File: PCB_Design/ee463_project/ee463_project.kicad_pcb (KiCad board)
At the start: 2 copper layers, 159.3 x 123.2 mm, 25 parts, among them Q1 C2M0080120D, U1 TLP250, U2 L7808, U3 ACS712xLCTR-30A

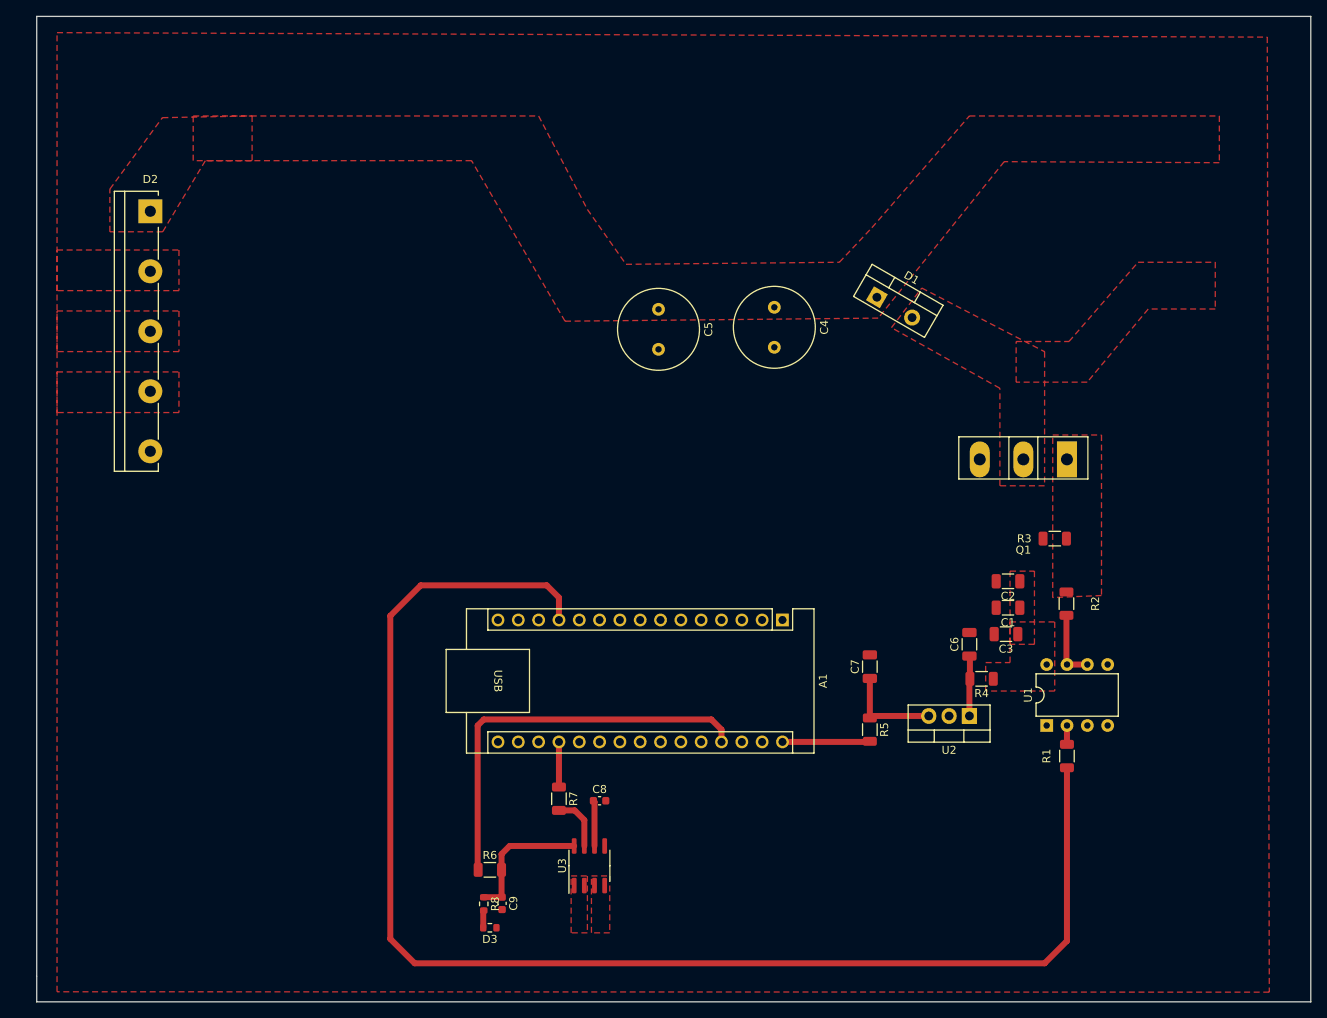
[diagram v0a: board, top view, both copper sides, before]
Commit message: PCB Design Updated
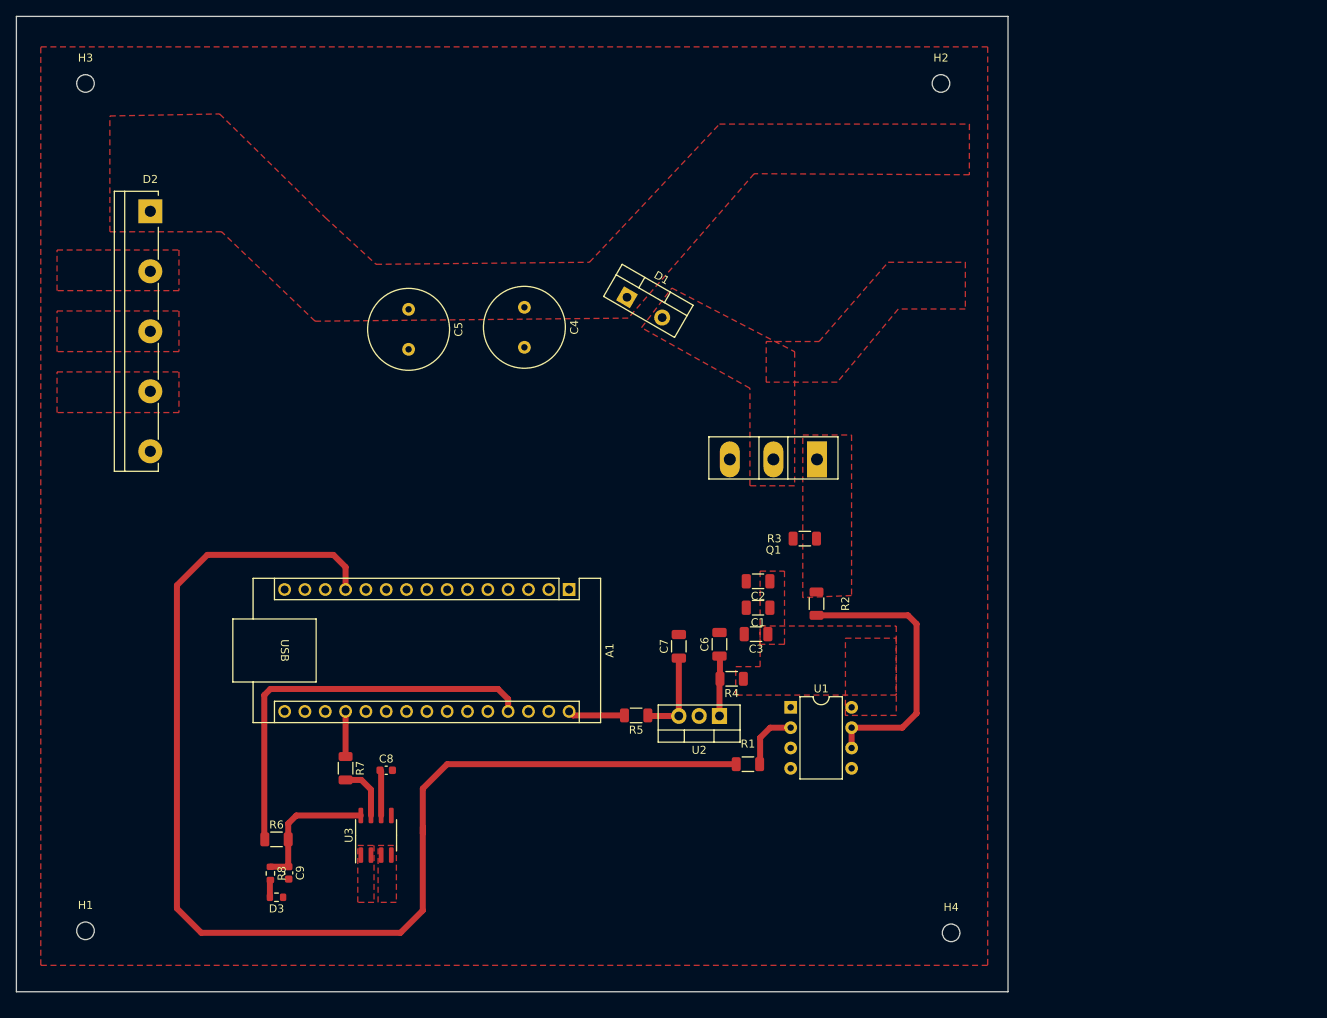
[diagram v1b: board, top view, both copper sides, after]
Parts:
- added H1: MountingHole, MountingHole:MountingHole_2.2mm_M2, F.Cu at (54.4, 133.4)
- added H2: MountingHole, MountingHole:MountingHole_2.2mm_M2, F.Cu at (161.3, 27.4)
- added H3: MountingHole, MountingHole:MountingHole_2.2mm_M2, F.Cu at (54.4, 27.4)
- added H4: MountingHole, MountingHole:MountingHole_2.2mm_M2, F.Cu at (162.6, 133.6)
- moved R1 39.9 mm to (137.2, 112.5), turned to 0 degrees
- moved U1 32.1 mm to (142.5, 105.4), turned to 0 degrees
- moved C3 31.2 mm to (138.2, 96.3)
- moved Q1 31.2 mm to (145.8, 74.4)
- moved R3 31.2 mm to (144.3, 84.3)
- moved R4 31.2 mm to (135.1, 101.9)
- moved C1 31.2 mm to (138.4, 93.0)
- moved C2 31.2 mm to (138.4, 89.7)
- moved C4 31.2 mm to (109.2, 55.4)
- moved C5 31.2 mm to (94.7, 55.7)
- moved C6 31.2 mm to (133.6, 97.5)
- moved D1 31.2 mm to (122.0, 54.2)
- moved R2 31.2 mm to (145.7, 92.5)
- moved U2 31.2 mm to (133.6, 106.5)
- moved R5 29.3 mm to (123.2, 106.4), turned to 180 degrees
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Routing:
- net Net-(R2-Pad1): track 8.72 -> 35.5 mm
- net PWM: track 175.1 -> 156.1 mm
- net Net-(R1-Pad2): track 2.36 -> 7.67 mm
- net V_in_arduino: track 11.0 -> 7.13 mm
- net Net-(C7-Pad1): track 12.4 -> 11.1 mm
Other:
- board size 159.3 x 123.2 mm -> 124 x 121.9 mm
